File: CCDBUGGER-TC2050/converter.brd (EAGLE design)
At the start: 30.5 x 72.9 mm, 13 parts

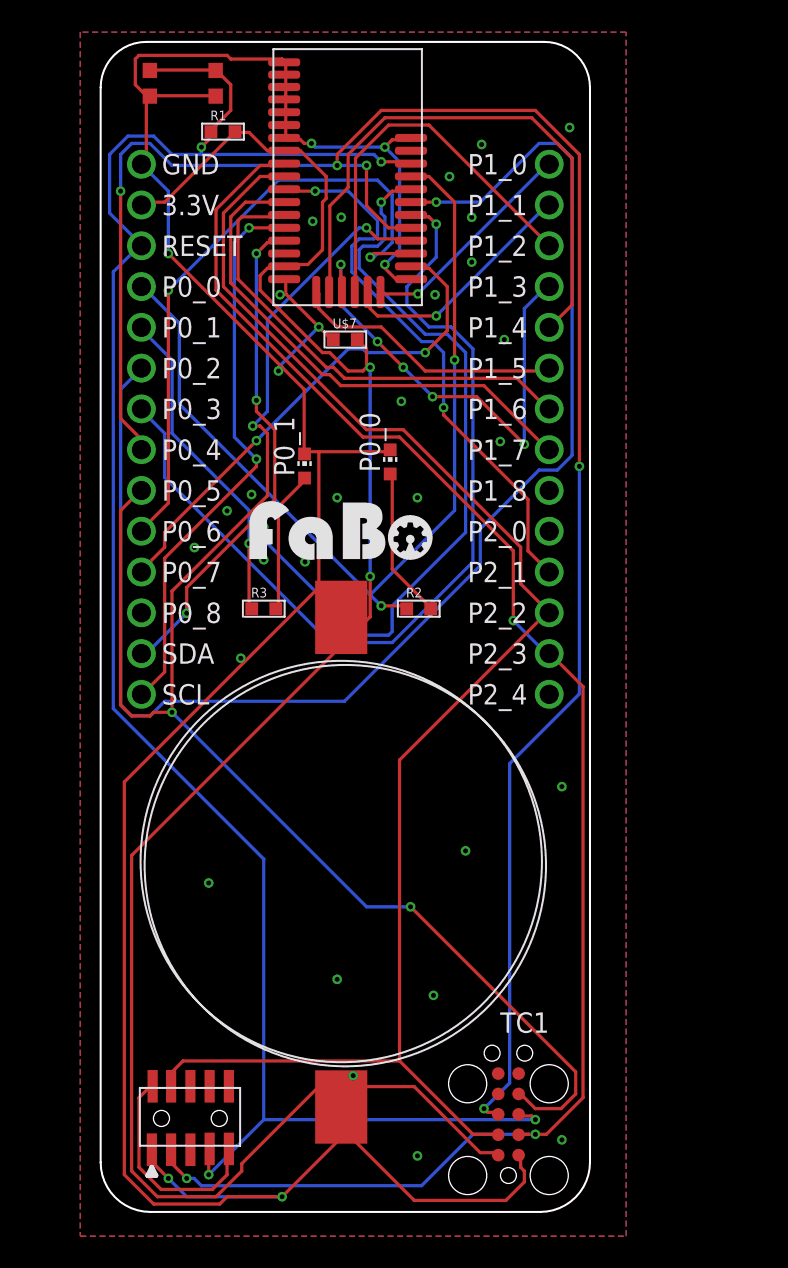
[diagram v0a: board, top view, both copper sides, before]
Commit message: Add update
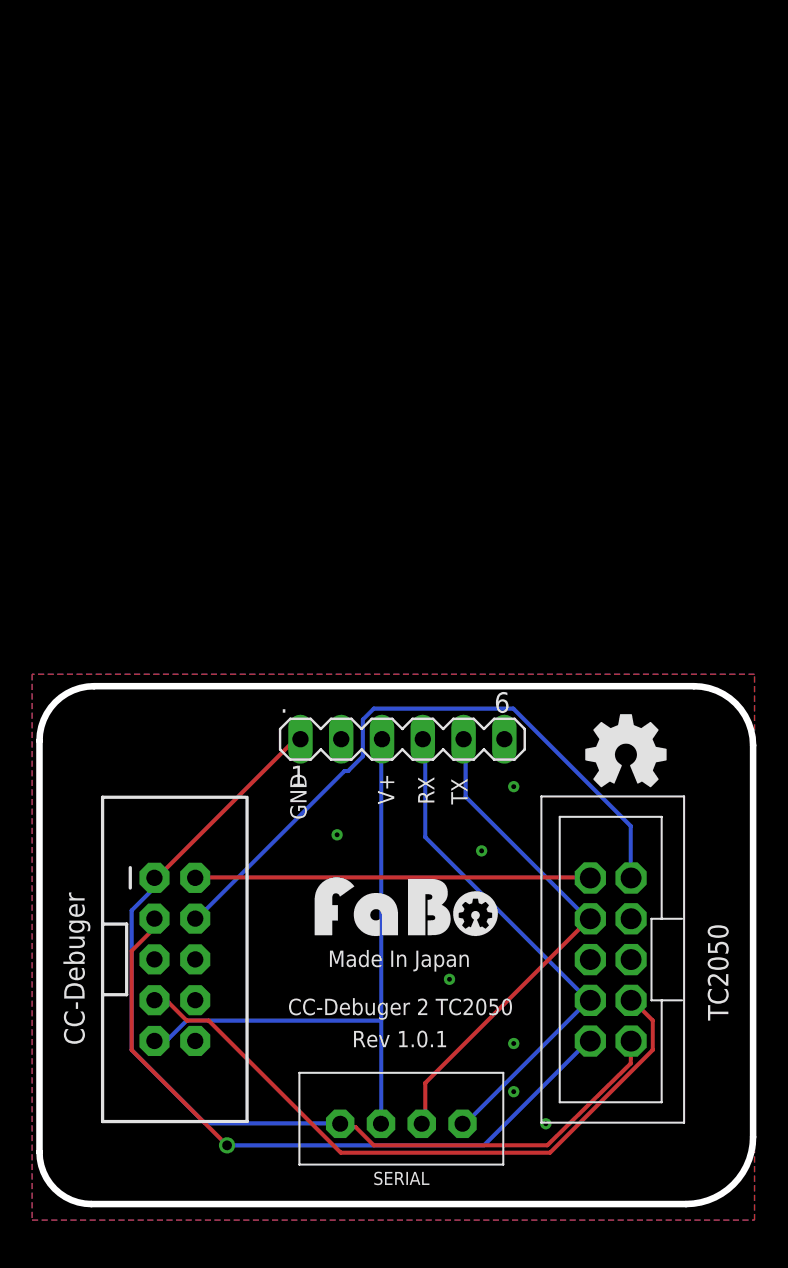
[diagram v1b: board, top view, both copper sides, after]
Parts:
- removed P0_0, P0_1: (no value), led:CHIP-LED0603
- removed R1: 10K, GClue-Resistors:0603
- removed R2, R3: 180, GClue-Resistors:0603
- removed TC1: TC2050-IDCB, TagConnect:TC2050-IDC
- removed U$3: BLUEGIGA-BLE113, GClueBT:BLUEGIGA-BLE113
- removed U$5: SWICTH-4P(KMR2), gclue-test:SWITCH-4P(KMR2)
- removed U$7: CAPACITOR0603, GClue-Capacitor:0603
- removed U$8: (no value), FaBo:LOGO_FABO_M
- added .: (no value), con-lstb:MA06-1
- added JP1: M05X2SHD, SparkFun-Connectors:2X5-SHROUDED
- added SERIAL: (no value), FaBo-Template:FABO_BRICK_SERIAL_CONNECTOR_I
- U$1: value PIN-HEADER-SMT(1.27MM)2X5 -> (none); device gclue:PIN-HEADER-SMT(1.27MM)2X5 -> FaBo:LOGO_FABO_M
- U$2: value BREAKOUT_BLE -> (none); device gclue:BREAKOUT_BLE -> FaBo-etc:LOGO_OSHW_M
- U$4: value SMTU2450-TOP -> TC-2050-SOCKET; device GClue-Supply:SMTU2450 -> GClue-Debbuger:TC-2050-SOCKET
- moved U$2 29.8 mm to (34.0, 28.0)
- moved U$1 17.6 mm to (20.3, 16.7)
- moved U$4 16.9 mm to (33.0, 19.0)
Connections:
- removed net +3V3: U$1.2, U$1.9
- removed net N$12: U$2.P0_8
- removed net P0_0: R2.1, U$2.P0_0, U$3.33
- removed net P0_1: R3.1, U$2.P0_1, U$3.32
- removed net P0_2: U$2.P0_2, U$3.31
- removed net P0_3: U$2.P0_3, U$3.30
- removed net P0_4: TC1.6, U$2.P0_4, U$3.29
- removed net P0_5: TC1.7, U$2.P0_5, U$3.28
- removed net P0_6: U$2.P0_6, U$3.27
- removed net P0_7: U$2.P0_7, U$3.26
- removed net P1_0: U$2.P1_0, U$3.24
- removed net P1_1: U$2.P1_1, U$3.23
- removed net P1_2: U$2.P1_2, U$3.22
- removed net P1_3: U$2.P1_3, U$3.21
- removed net P1_4: U$2.P1_4, U$3.20
- removed net P1_5: U$2.P1_5, U$3.19
- removed net P1_6: U$2.P1_6, U$3.13
- removed net P1_7: U$2.P1_7, U$3.12
- removed net P1_8: U$2.P1_8
- removed net P1_9: U$2.P2_0
- removed net P2_0: U$2.P2_1, U$3.11
- removed net R1: P0_1.A, R3.2
- removed net R2: P0_0.A, R2.2
- removed net SCL: U$2.SCL, U$3.14
- removed net SDA: U$2.SDA, U$3.15
- new net 3V3: ..3, JP1.9, SERIAL.VCC
- new net CSN: JP1.5
- new net MISO: JP1.10
- new net MOSI: JP1.8
- new net RX: ..4, SERIAL.RX, U$4.7
- new net SCLK: JP1.6
- new net TX: ..5, SERIAL.TX, U$4.6
- net 3.3V: now also JP1.2, U$4.2; no longer R1.2, TC1.2, U$2.3.3V, U$3.17, U$3.8, U$4.P$_VCC, U$7.2
- net DEBUG_CLOCK: now also JP1.4, U$4.4; no longer TC1.4, U$1.4, U$2.P2_2, U$3.10
- net DEBUG_DATA: now also JP1.3, U$4.3; no longer TC1.3, U$1.3, U$2.P2_3, U$3.9
- net GND: now also ..1, JP1.1, SERIAL.GND, U$4.1; no longer P0_0.C, P0_1.C, TC1.1, U$1.1, U$2.GND, U$3.1, U$3.18, U$3.2, U$3.25, U$3.3, U$3.36, U$3.4, U$3.5, U$3.6, U$3.7, U$4.P$_GND, U$5.3, U$5.4, U$7.1
- net RESET: now also JP1.7, U$4.5; no longer R1.1, TC1.5, U$1.7, U$2.RESET, U$3.34, U$5.1, U$5.2
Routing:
- net P0_4: track 121.9 -> 0.00 mm, vias 5 -> 0
- net GND: track 176.3 -> 61.1 mm, vias 36 -> 7
- net 3.3V: track 123.0 -> 24.6 mm, vias 2 -> 0
- net P0_5: track 97.2 -> 0.00 mm, vias 4 -> 0
- net P0_2: track 88.4 -> 0.00 mm, vias 1 -> 0
- net RESET: track 120.8 -> 41.3 mm, vias 4 -> 0
- net P0_1: track 67.4 -> 0.00 mm, vias 2 -> 0
- net DEBUG_DATA: track 102.1 -> 42.5 mm, vias 3 -> 1
- net P0_0: track 57.8 -> 0.00 mm, vias 2 -> 0
- net P0_3: track 56.5 -> 0.00 mm, vias 1 -> 0
- net DEBUG_CLOCK: track 94.6 -> 40.1 mm
- net P0_6: track 40.2 -> 0.00 mm, vias 2 -> 0
- net 3V3: track 0.00 -> 38.6 mm
- net P1_4: track 36.1 -> 0.00 mm
- net P2_0: track 35.2 -> 0.00 mm, vias 2 -> 0
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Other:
- board size 30.5 x 72.9 mm -> 44.4 x 32.3 mm
- board text added: "CC-Debuger"
- board text added: "CC-Debuger 2 TC2050"
- board text added: "GND"
- board text added: "Made In Japan"
- board text added: "RX"
- board text added: "Rev 1.0.1"
- board text added: "TC2050"
- board text added: "TX"
- board text added: "V+"
- board text removed: "Rev.Beat20150902"
